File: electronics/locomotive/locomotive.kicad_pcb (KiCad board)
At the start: 2 copper layers, 16 x 64 mm, 0 parts

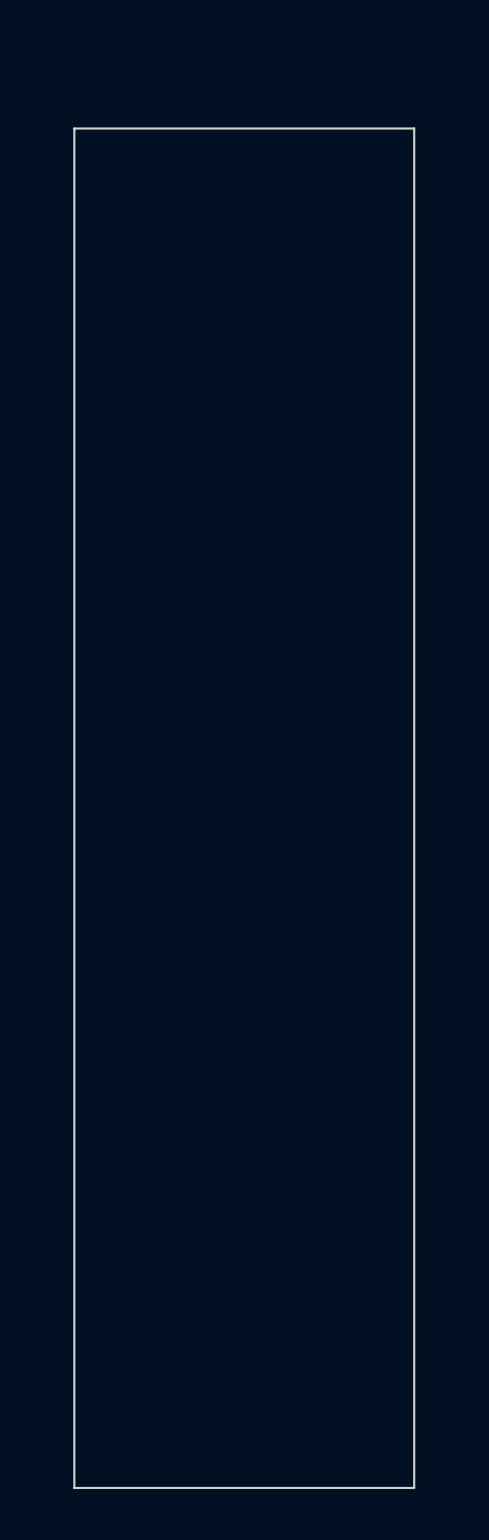
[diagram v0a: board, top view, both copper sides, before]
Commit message: electronics: locomotive: Board Rev 1.0
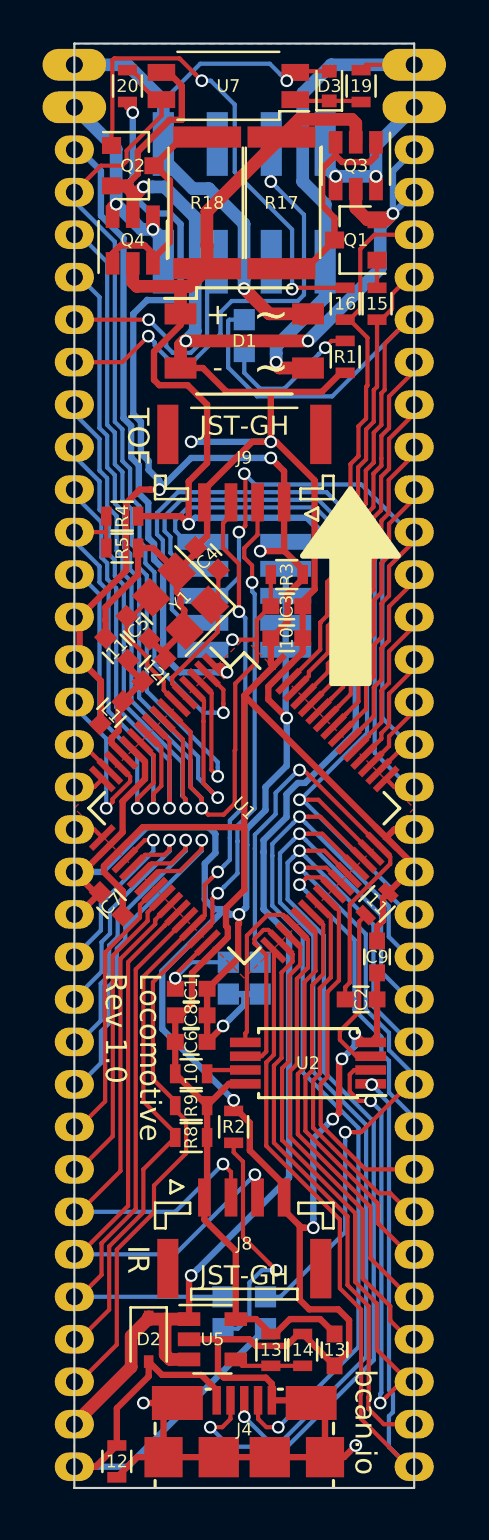
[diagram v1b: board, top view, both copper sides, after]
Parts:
- added 10: 100n, Capacitors_SMD:C_0603, F.Cu at (152.0, 92.0)
- added 10: 10k, Resistors_SMD:R_0603, F.Cu at (147.5, 112.5)
- added 11: 100n, Capacitors_SMD:C_0603, F.Cu at (144.0, 92.5)
- added 11: 10k, Resistors_SMD:R_0603, F.Cu at (156.2, 104.5)
- added 12: 10k, Resistors_SMD:R_0603, F.Cu at (144.0, 130.8)
- added 12: 1u, Capacitors_SMD:C_0603, F.Cu at (145.8, 93.5)
- added 13: 2u2, Capacitors_SMD:C_0603, F.Cu at (154.2, 125.5)
- added 13: 33k2, Resistors_SMD:R_0603, F.Cu at (151.2, 125.5)
- added 14: 26k1, Resistors_SMD:R_0603, F.Cu at (152.8, 125.5)
- added 15: 1k, Resistors_SMD:R_0603, F.Cu at (156.2, 76.2)
- added 16: 1k, Resistors_SMD:R_0603, F.Cu at (154.8, 76.2)
- added 19: 1k5, Resistors_SMD:R_0603, F.Cu at (155.5, 66.0)
- added 20: 10k, Resistors_SMD:R_0603, F.Cu at (144.5, 66.0)
- added C1: 2u2, Capacitors_SMD:C_0603, F.Cu at (147.5, 108.5)
- added C2: 2u2, Capacitors_SMD:C_0603, F.Cu at (155.5, 109.0)
- added C3: 100n, Capacitors_SMD:C_0603, F.Cu at (152.0, 90.5)
- added C4: 10p, Capacitors_SMD:C_0603, F.Cu at (148.2, 88.2)
- added C5: 10p, Capacitors_SMD:C_0603, F.Cu at (145.0, 91.5)
- added C6: 4u7, Capacitors_SMD:C_0603, F.Cu at (147.5, 111.0)
- added C7: 100n, Capacitors_SMD:C_0603, F.Cu at (143.8, 104.5)
- added C8: 100n, Capacitors_SMD:C_0603, F.Cu at (147.5, 109.8)
- added C9: 100n, Capacitors_SMD:C_0603, F.Cu at (156.2, 107.0)
- added D1: CDBHM240L-HF, bcan:TO-269AA, F.Cu at (150.0, 78.0)
- added D2: CUS08F30, Diodes_SMD:D_SOD-323, F.Cu at (145.5, 125.0)
- added D3: 1N4148, Diodes_SMD:D_SOD-523, F.Cu at (154.0, 66.0)
- added J1: PIN[1..32], bcan:Castellations_1x32_Pitch2.00mm, F.Cu at (142.0, 69.0)
- added J2: PIN[33..64], bcan:Castellations_1x32_Pitch2.00mm, F.Cu at (158.0, 131.0)
- added J3: JTAG, Pin_Headers:Pin_Header_Straight_2x05_Pitch1.27mm_SMD, B.Cu at (150.0, 90.0)
- added J4: USB_OTG, bcan:USB_Micro-B_Amphenol_10118192, F.Cu at (150.0, 130.6)
- added J5: RAILS, bcan:Castellations_1x02_Pitch2.00mm, F.Cu at (142.0, 65.0)
- added J6: MOTOR, bcan:Castellations_1x02_Pitch2.00mm, F.Cu at (158.0, 67.0)
- added J7: TRAIN, Pin_Headers:Pin_Header_Straight_2x04_Pitch2.54mm_SMD, B.Cu at (150.0, 71.5)
- added J8: IR, Connectors_JST:JST_GH_BM04B-GHS-TBT_04x1.25mm_Straight, F.Cu at (150.0, 120.0)
- added J9: TOF, Connectors_JST:JST_GH_SM04B-GHS-TB_04x1.25mm_Angled, F.Cu at (150.0, 84.0)
- added JP1: BOOT0, bcan:Solder_Jumper_NC, B.Cu at (150.0, 77.8)
- added JP2: BOOT1, bcan:Solder_Jumper_NC, B.Cu at (149.0, 123.8)
- added JP3: VCAP1, bcan:Solder_Jumper_NO, B.Cu at (149.2, 108.0)
- added JP4: VCAP2, bcan:Solder_Jumper_NO, B.Cu at (150.8, 108.0)
- added JP5: USB_VBUS, bcan:Solder_Jumper_NC, B.Cu at (151.0, 123.8)
- added L1: 600, Capacitors_SMD:C_0603, F.Cu at (143.8, 95.5)
- added Q1: MMBT2222A, TO_SOT_Packages_SMD:SOT-23, F.Cu at (155.2, 73.2)
- added Q2: MMBT2222A, TO_SOT_Packages_SMD:SOT-23, F.Cu at (144.8, 69.8)
- added Q3: DMG6601LVT, TO_SOT_Packages_SMD:SOT-23-6, F.Cu at (155.2, 69.8)
- added Q4: DMG6601LVT, TO_SOT_Packages_SMD:SOT-23-6, F.Cu at (144.8, 73.2)
- added R1: 10k, Resistors_SMD:R_0603, F.Cu at (154.8, 78.8)
- added R17: 100, Resistors_SMD:R_2512, F.Cu at (151.8, 71.5)
- added R18: 100, Resistors_SMD:R_2512, F.Cu at (148.2, 71.5)
- added R2: 10k, Resistors_SMD:R_0603, F.Cu at (149.5, 115.0)
- added R3: 10k, Resistors_SMD:R_0603, F.Cu at (152.0, 89.0)
- added R4: 13k3, Resistors_SMD:R_0603, F.Cu at (144.2, 86.2)
- added R5: 2k8, Resistors_SMD:R_0603, F.Cu at (144.2, 87.8)
- added R8: 4k7, Resistors_SMD:R_0603, F.Cu at (147.5, 115.5)
- added R9: 4k7, Resistors_SMD:R_0603, F.Cu at (147.5, 114.0)
- added U1: STM32F405RGTx, Housings_QFP:TQFP-64_10x10mm_Pitch0.5mm, F.Cu at (150.0, 100.0)
- added U2: M95512-RDW6TP, Housings_SSOP:TSSOP-8_4.4x3mm_Pitch0.65mm, F.Cu at (153.0, 112.0)
- added U5: SPX3819M5, TO_SOT_Packages_SMD:SOT-23-5, F.Cu at (148.5, 125.0)
- added U7: TLP293, Housings_SSOP:SOP-4_4.4x2.8mm_Pitch1.27mm, F.Cu at (149.2, 66.0)
- added Y1: 16MHz, Crystals:Crystal_SMD_3225-4pin_3.2x2.5mm, F.Cu at (147.0, 90.2)
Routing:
- net GND: track 0.00 -> 222.6 mm, vias 0 -> 16
- net 2V8: track 0.00 -> 124.7 mm, vias 0 -> 4
- net VCC: track 0.00 -> 93.9 mm, vias 0 -> 2
- net PA10: track 0.00 -> 51.8 mm, vias 0 -> 2
- net PA11: track 0.00 -> 48.7 mm, vias 0 -> 2
- net PA12: track 0.00 -> 47.3 mm, vias 0 -> 2
- net PB11: track 0.00 -> 47.1 mm, vias 0 -> 2
- net PB12: track 0.00 -> 46.7 mm, vias 0 -> 1
- net PB10: track 0.00 -> 45.0 mm, vias 0 -> 2
- net PB14: track 0.00 -> 43.8 mm, vias 0 -> 2
- net NRST: track 0.00 -> 42.8 mm, vias 0 -> 2
- net PC13: track 0.00 -> 39.1 mm, vias 0 -> 1
- net PA13: track 0.00 -> 37.5 mm, vias 0 -> 1
- net PB13: track 0.00 -> 35.1 mm
- net BOOT0: track 0.00 -> 33.8 mm
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- added copper zone on F.Cu, net 2V8
- added copper zone on B.Cu, net GND
- added copper zone on F.Cu, net GND
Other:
- board size 16 x 64 mm -> 16 x 68 mm
- net class Default: clearance 0.2 -> 0.16; trace_width 0.25 -> 0.2
- net class Motor added: clearance 0.16, trace_width 0.6, via_dia 0.6, via_drill 0.4
- net class Power added: clearance 0.16, trace_width 0.3, via_dia 0.6, via_drill 0.4
- rule trace_clearance: 0.2 -> 0.16
- board text added: "+"
- board text added: "-"
- board text added: "2V8"
- board text added: "5V"
- board text added: "B8"
- board text added: "B9"
- board text added: "BOOT0"
- board text added: "BOOT1"
- board text added: "C13"
- board text added: "C14"
- board text added: "C15"
- board text added: "F-"
- board text added: "GND"
- board text added: "IR"
- board text added: "JST-GH"
- board text added: "JTAG"
- board text added: "L"
- board text added: "Locomotive Rev 1.0"
- board text added: "MOTOR"
- board text added: "NRST"
- board text added: "PA0"
- board text added: "PA1"
- board text added: "PA10"
- board text added: "PA11"
- board text added: "PA12"
- board text added: "PA13"
- board text added: "PA14"
- board text added: "PA15"
- board text added: "PA2"
- board text added: "PA3"
- board text added: "PA4"
- board text added: "PA5"
- board text added: "PA6"
- board text added: "PA7"
- board text added: "PA8"
- board text added: "PA9"
- board text added: "PB0"
- board text added: "PB1"
- board text added: "PB10"
- board text added: "PB11"
- board text added: "PB12"
- board text added: "PB13"
- board text added: "PB14"
- board text added: "PB15"
- board text added: "PB2"
- board text added: "PB3"
- board text added: "PB4"
- board text added: "PB5"
- board text added: "PB6"
- board text added: "PB7"
- board text added: "PC0"
- board text added: "PC1"
- board text added: "PC10"
- board text added: "PC11"
- board text added: "PC12"
- board text added: "PC2"
- board text added: "PC3"
- board text added: "PC4"
- board text added: "PC5"
- board text added: "PC6"
- board text added: "PC7"
- board text added: "PC8"
- board text added: "PC9"
- board text added: "PD2"
- board text added: "R"
- board text added: "R-"
- board text added: "RAILS"
- board text added: "TOF"
- board text added: "VBAT"
- board text added: "VCAP"
- board text added: "VCC"
- board text added: "bcan.io"
